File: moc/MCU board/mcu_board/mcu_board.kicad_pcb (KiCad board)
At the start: 2 copper layers, 41 x 30 mm, 10 parts, among them J1 Conn_01x04_Female, J2 Conn_01x05_Female, J3 Conn_01x05_Male, J4 Conn_01x09_Female, J5 Conn_01x09_Female, U1 ATtiny861V-10SU

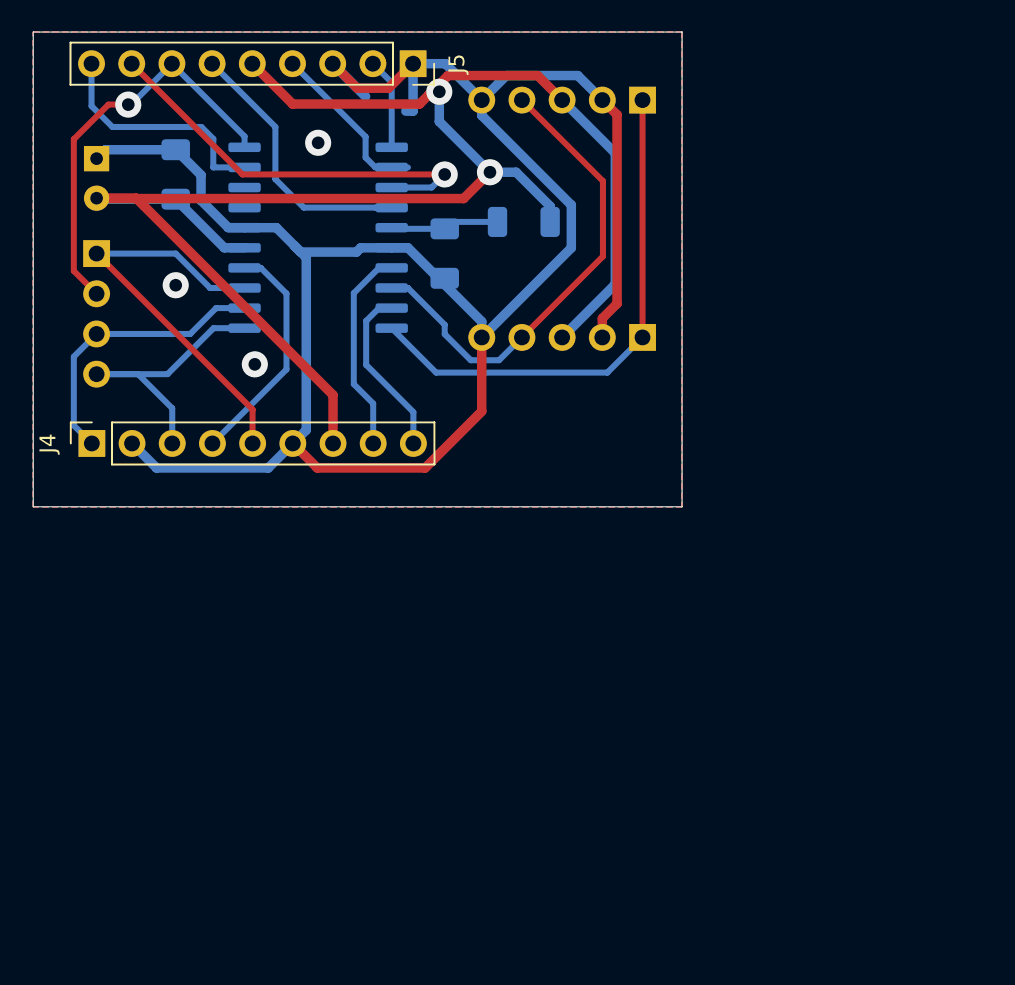
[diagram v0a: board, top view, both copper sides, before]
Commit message: first protoype
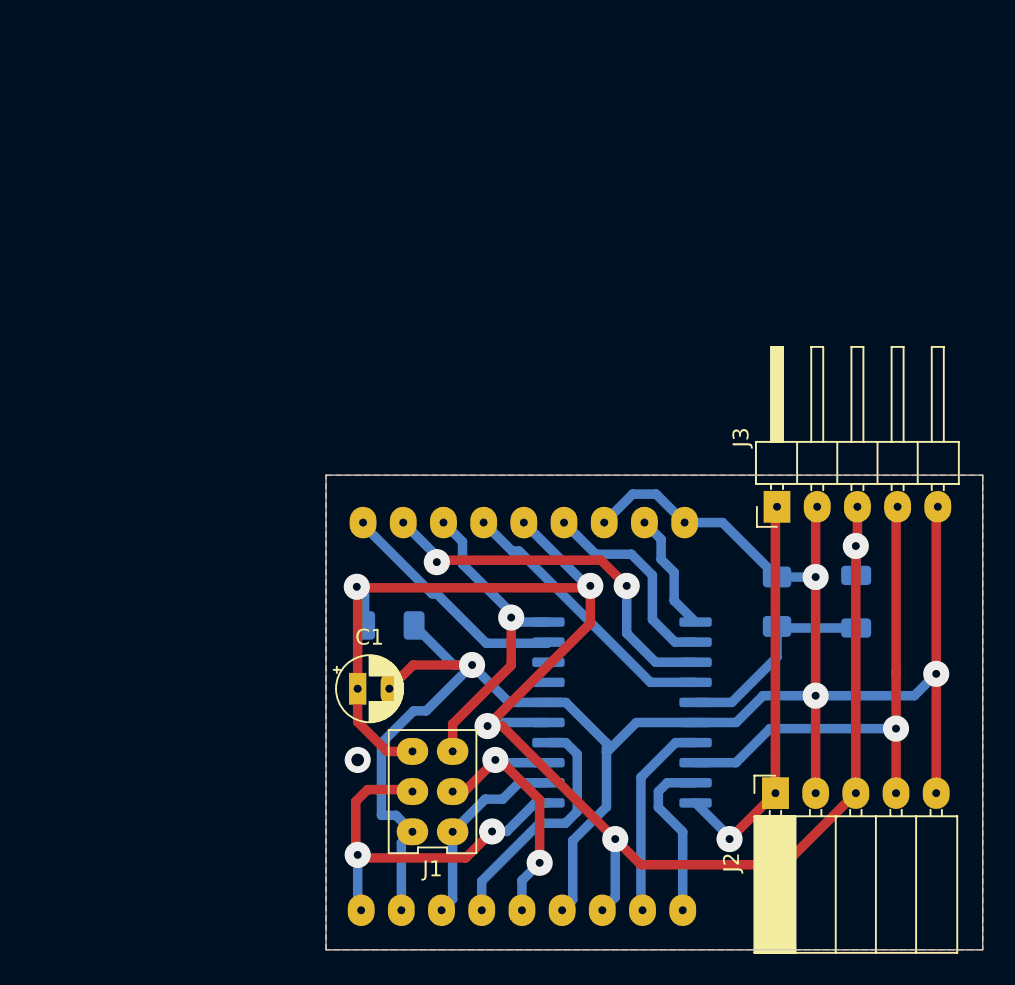
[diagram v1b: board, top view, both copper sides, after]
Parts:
- C1: footprint Capacitor_THT:CP_Radial_Tantal_D5.0mm_P2.50mm -> Capacitor_THT:CP_Radial_D4.0mm_P1.50mm; moved to F.Cu
- J1: value Conn_01x04_Female -> Conn_02x03_Counter_Clockwise; footprint Connector_PinSocket_2.54mm:PinSocket_1x04_P2.54mm_Vertical -> .Ambisonic:ICSP_Header_P2.54_SelfSolder; moved to F.Cu
- J2, J3: moved to F.Cu
- J4, J5: footprint Connector_PinSocket_2.54mm:PinSocket_1x09_P2.54mm_Vertical -> .Ambisonic:Header-01x09-p2.54-selfsolder; moved to B.Cu
- moved J4 40.1 mm to (106.9, 122.5), turned to 0 degrees
- moved J1 40.1 mm to (101.2, 115.0), turned to 90 degrees
- moved C1 37.3 mm to (96.5, 108.5), turned to 0 degrees
- moved U1 35.6 mm to (113.2, 110.0)
- moved L1 31.9 mm to (128.0, 103.0), turned to -90 degrees
- moved C2 31.5 mm to (98.5, 104.5), turned to 180 degrees
- moved C3 30.4 mm to (123.0, 103.0), turned to -90 degrees
- moved J2 30.0 mm to (122.9, 115.1)
- moved J5 29.8 mm to (107.0, 98.0), turned to 180 degrees
- moved J3 27.1 mm to (123.0, 97.0)
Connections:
- net PB1 renamed BUT1
- net PB2 renamed BUT2
- net PB3 renamed BUT3
- C1 pad 1: GND -> VCC
- C1 pad 2: VCC -> GND
- J1 pad 1: PSFHCLK -> MISO
- J1 pad 2: ENCB -> PSFHCLK
- J1 pad 3: MISO -> ENCB
- J1 pad 4: MOSI -> VCC
- J4 pad 1: MISO -> BUT0
- J4 pad 3: MOSI -> MISO
- U1 pad 1: MOSI -> BUT0
- U1 pad 7: (no net) -> unconnected-(U1-Pad7)
- U1 pad 8: (no net) -> unconnected-(U1-Pad8)
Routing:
- net BUT0: track 0.00 -> 24.5 mm, vias 0 -> 2
- net MOSI: track 18.4 -> 0.00 mm
- net GND: track 137.0 -> 128.5 mm, vias 3 -> 5
- net PSFHCLK: track 26.3 -> 18.3 mm, vias 0 -> 2
- net SDA: track 32.9 -> 25.4 mm, vias 0 -> 1
- net VCC: track 111.3 -> 105.0 mm, vias 2 -> 5
- net Net-(C3-Pad2): track 7.21 -> 13.3 mm
- net ENCB: track 25.7 -> 20.2 mm
- net MISO: track 18.0 -> 12.6 mm
- net ADC0: track 10.8 -> 13.1 mm
- net ENCSW: track 26.4 -> 24.2 mm, vias 1 -> 2
- net ADC1: track 5.78 -> 7.62 mm
- net SCL: track 30.3 -> 31.7 mm, vias 0 -> 1
- net PSHFUPDATE: track 14.7 -> 15.5 mm
- net BUT1: track 18.1 -> 17.6 mm
- removed copper zone on F.Cu, net (none)
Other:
- board size 41 x 30 mm -> 41.5 x 30 mm
- net class Default removed
- net class VCC removed
